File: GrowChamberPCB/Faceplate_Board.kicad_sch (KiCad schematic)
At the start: 23 parts, among them J11 Conn_01x26_Pin, J12 Fogger Fill Solenoid, J13 Drain Solenoid, J14 Glycol Solenoid, J15 Fogger Disc, J16 Fogger Float, J17 Drain Level, J18 Heater Fans Con, J19 Soil Moisture 2, J20 Soil Moisture 3, J21 Soil Moisture 1, J22 Fan Connector, J23 SCD30 Connector, J24 LED_Con, J25 Screw_Terminal_01x02, J4 Glycol Fans, J5 Circ Fans, J6 UART, J9 Water Solenoid, SW3 BootSwitch, SW4 ResetButton, U7 PCA9555PW

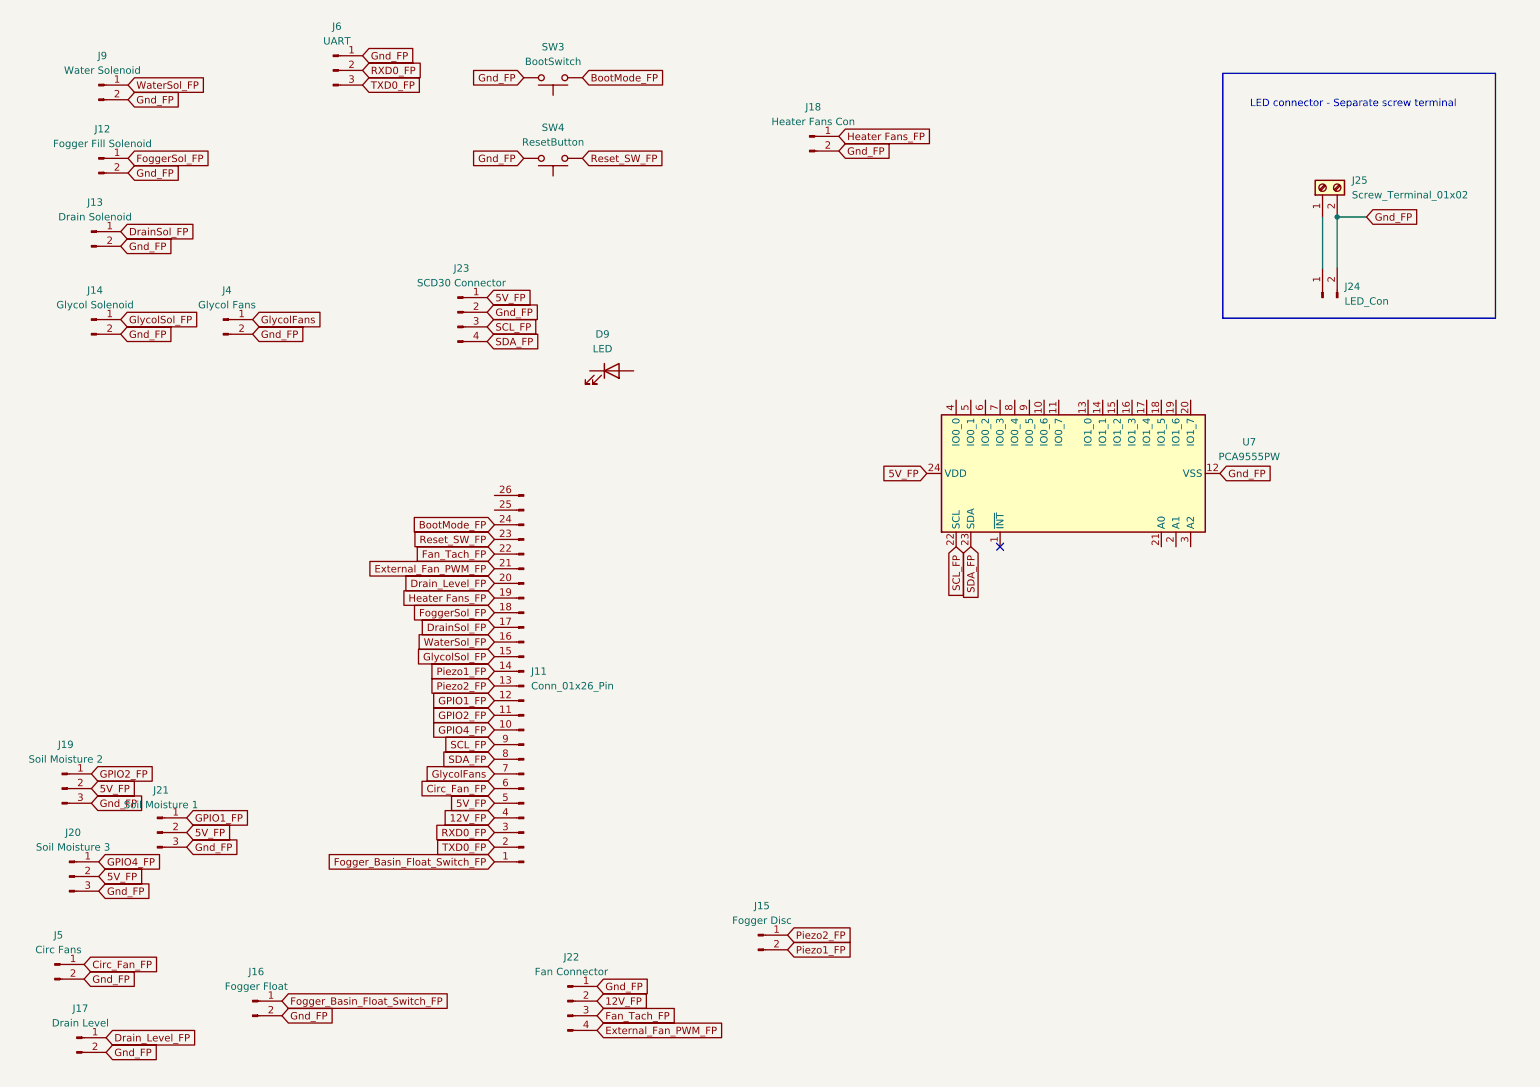
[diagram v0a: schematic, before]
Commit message: struggling to make BOM
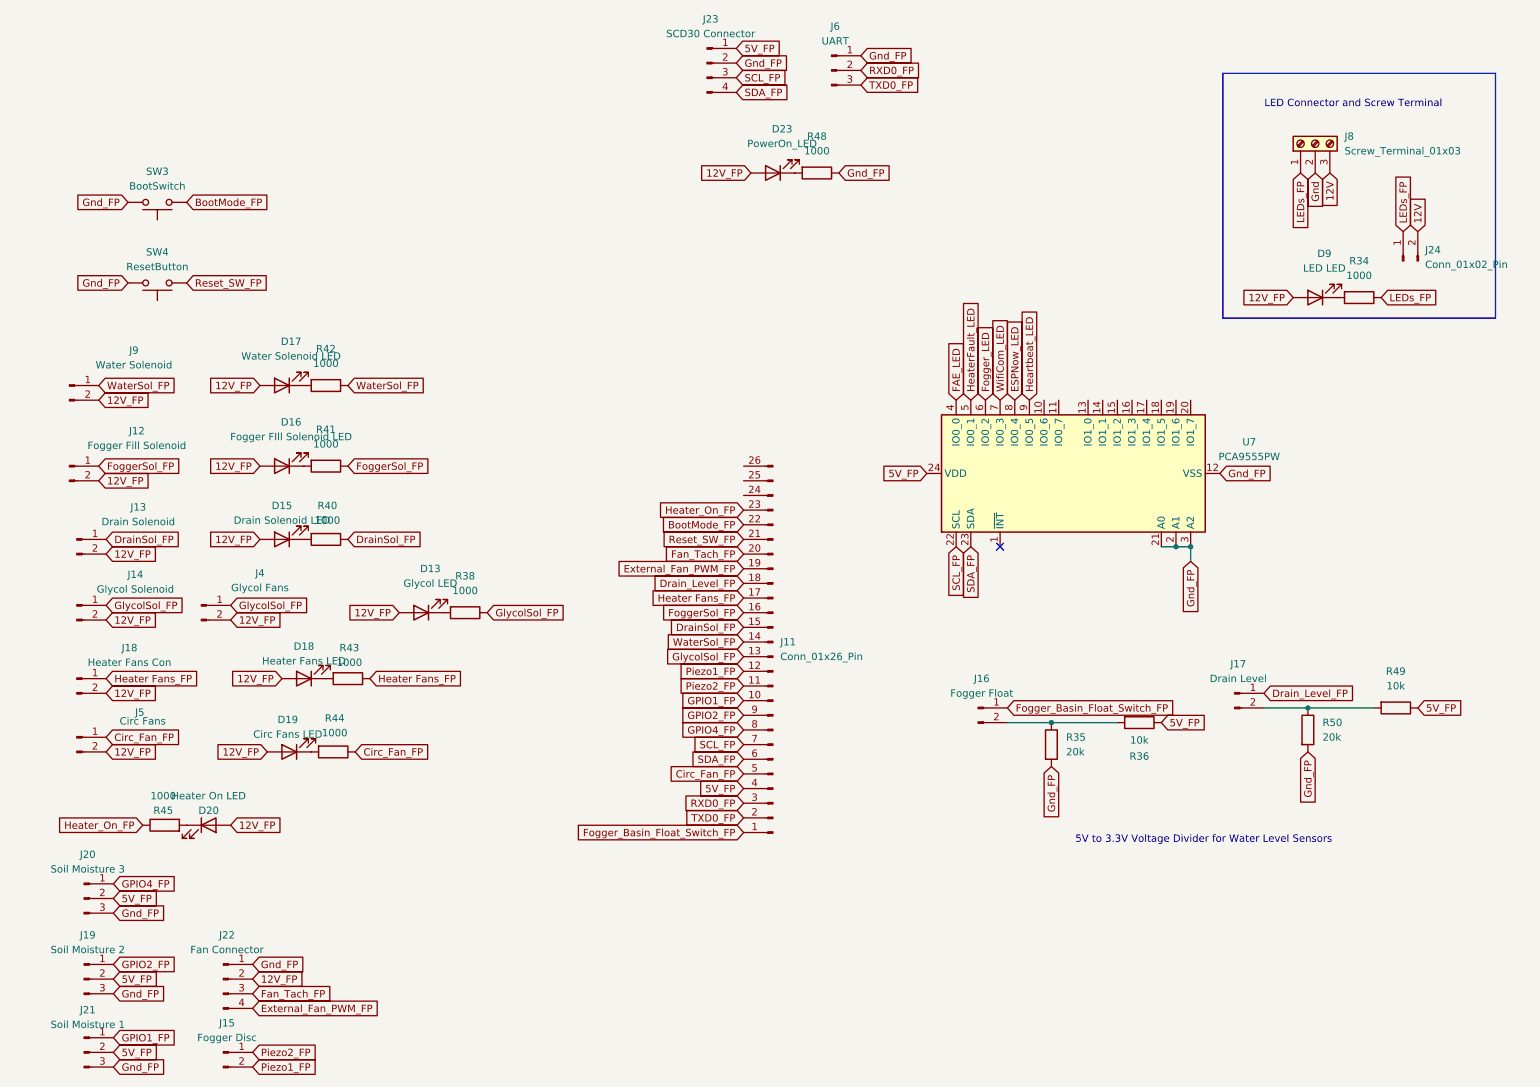
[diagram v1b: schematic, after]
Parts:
- removed J25: Screw_Terminal_01x02, symbol Connector:Screw_Terminal_01x02
- added D13: Glycol LED, symbol Device:LED
- added D15: Drain Solenoid LED, symbol Device:LED
- added D16: Fogger FIll Solenoid LED, symbol Device:LED
- added D17: Water Solenoid LED, symbol Device:LED
- added D18: Heater Fans LED, symbol Device:LED
- added D19: Circ Fans LED, symbol Device:LED
- added D20: Heater On LED, symbol Device:LED
- added D23: PowerOn_LED, symbol Device:LED
- added J8: Screw_Terminal_01x03, symbol Connector:Screw_Terminal_01x03
- added R34, R38, R40, R41, R42, R43, R44, R45, R48: 1000, symbol Device:R
- added R35, R50: 20k, symbol Device:R
- added R36, R49: 10k, symbol Device:R
- D9: value LED -> LED LED
- J19, J20, J21, J6: footprint Connector_Molex:Molex_KK-254_AE-6410-03A_1x03_P2.54mm_Vertical -> (none)
- J24: value LED_Con -> Conn_01x02_Pin
- U7: footprint Package_SO:TSSOP-24_4.4x7.8mm_P0.65mm -> (none)
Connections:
- net 12V_FP: now also D9.2 (A), J12.2 (Pin_2), J13.2 (Pin_2), J14.2 (Pin_2), J18.2 (Pin_2), J4.2 (Pin_2), J5.2 (Pin_2), J9.2 (Pin_2), D13.2 (A), D15.2 (A), D16.2 (A), D17.2 (A), D18.2 (A), D19.2 (A), D20.2 (A), D23.2 (A); no longer J11.4 (Pin_4)
- net 5V_FP: now also J11.4 (Pin_4), R36.1, R49.1; no longer J11.5 (Pin_5)
- net BootMode_FP: now also J11.22 (Pin_22); no longer J11.24 (Pin_24)
- net Circ_Fan_FP: now also J11.5 (Pin_5), R44.1; no longer J11.6 (Pin_6)
- net DrainSol_FP: now also J11.15 (Pin_15), R40.1; no longer J11.17 (Pin_17)
- net Drain_Level_FP: now also J11.18 (Pin_18); no longer J11.20 (Pin_20)
- net External_Fan_PWM_FP: now also J11.19 (Pin_19); no longer J11.21 (Pin_21)
- net Fan_Tach_FP: now also J11.20 (Pin_20); no longer J11.22 (Pin_22)
- net FoggerSol_FP: now also J11.16 (Pin_16), R41.1; no longer J11.18 (Pin_18)
- net GPIO1_FP: now also J11.10 (Pin_10); no longer J11.12 (Pin_12)
- net GPIO2_FP: now also J11.9 (Pin_9); no longer J11.11 (Pin_11)
- net GPIO4_FP: now also J11.8 (Pin_8); no longer J11.10 (Pin_10)
- net GlycolSol_FP: now also J11.13 (Pin_13), J4.1 (Pin_1), R38.1; no longer J11.15 (Pin_15)
- net Gnd_FP: now also U7.2 (A1), U7.21 (A0), U7.3 (A2), R35.2, R48.1, R50.2; no longer J12.2 (Pin_2), J13.2 (Pin_2), J14.2 (Pin_2), J16.2 (Pin_2), J17.2 (Pin_2), J18.2 (Pin_2), J24.2 (Pin_2), J4.2 (Pin_2), J5.2 (Pin_2), J9.2 (Pin_2)
- net Heater Fans_FP: now also J11.17 (Pin_17), R43.1; no longer J11.19 (Pin_19)
- net Piezo1_FP: now also J11.12 (Pin_12); no longer J11.14 (Pin_14)
- net Piezo2_FP: now also J11.11 (Pin_11); no longer J11.13 (Pin_13)
- net Reset_SW_FP: now also J11.21 (Pin_21); no longer J11.23 (Pin_23)
- net SCL_FP: now also J11.7 (Pin_7); no longer J11.9 (Pin_9)
- net SDA_FP: now also J11.6 (Pin_6); no longer J11.8 (Pin_8)
- net WaterSol_FP: now also J11.14 (Pin_14), R42.1; no longer J11.16 (Pin_16)
- net FAE_LED: now reaches U7.4 (IO0_0)
- net HeaterFault_LED: now reaches U7.5 (IO0_1)
- net Fogger_LED: now reaches U7.6 (IO0_2)
- net WifiCom_LED: now reaches U7.7 (IO0_3)
- net ESPNow_LED: now reaches U7.8 (IO0_4)
- net Heartbeat_LED: now reaches U7.9 (IO0_5)
- net LEDs_FP: now reaches J24.1 (Pin_1)
- net LEDs_FP: now also J8.1 (Pin_1), R34.1
- net at D9.1 (K): now also R34.2
- removed net GlycolFans: J11.7 (Pin_7), J4.1 (Pin_1)
- new net: J17.2 (Pin_2), R49.2, R50.1
- new net: D17.1 (K), R42.2
- new net: D16.1 (K), R41.2
- new net: D19.1 (K), R44.2
- new net: J16.2 (Pin_2), R35.1, R36.2
- new net: D13.1 (K), R38.2
- new net: D23.1 (K), R48.2
- new net: D20.1 (K), R45.2
- new net: D18.1 (K), R43.2
- new net: D15.1 (K), R40.2
- new net 12V: J24.2 (Pin_2), J8.3 (Pin_3)
- new net Gnd: J8.2 (Pin_2)
- new net Heater_On_FP: J11.23 (Pin_23), R45.1
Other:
- note added: "5V to 3.3V Voltage Divider for Water Level Sensors"
- note added: "LED Connector and Screw Terminal"
- note removed: "LED connector - Separate screw terminal"
- moved on the sheet: J11, J12, J13, J14, J15, J16, J17, J18, J19, J20, J21, J22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
